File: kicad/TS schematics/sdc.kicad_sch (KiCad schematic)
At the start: 23 parts, among them J22 Activation Logic, K2 EV200-HAANA, K3 EV200-HAANA, K4 EV200-HAANA, K5 PNC113BDA, SW1 LVMS, SW10 TSMP Interlock, SW11 Motor Controller HVP800 Inter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, SW12 PL00X-301-50 Interlock, SW13 PL00Y-301-50 Interlock, SW14 PL00X-301-50 Interlock, SW15 PL00Y-301-50 Interlock, SW16 MINIMSDF000F HVD Interlock, SW2 IMD, SW3 AMS, SW5 Cockpit Shutdown Button, SW6 Left Shutdown Button, SW7 Right Shutdown Button, SW8 Inertia Switch, SW9 BOTS

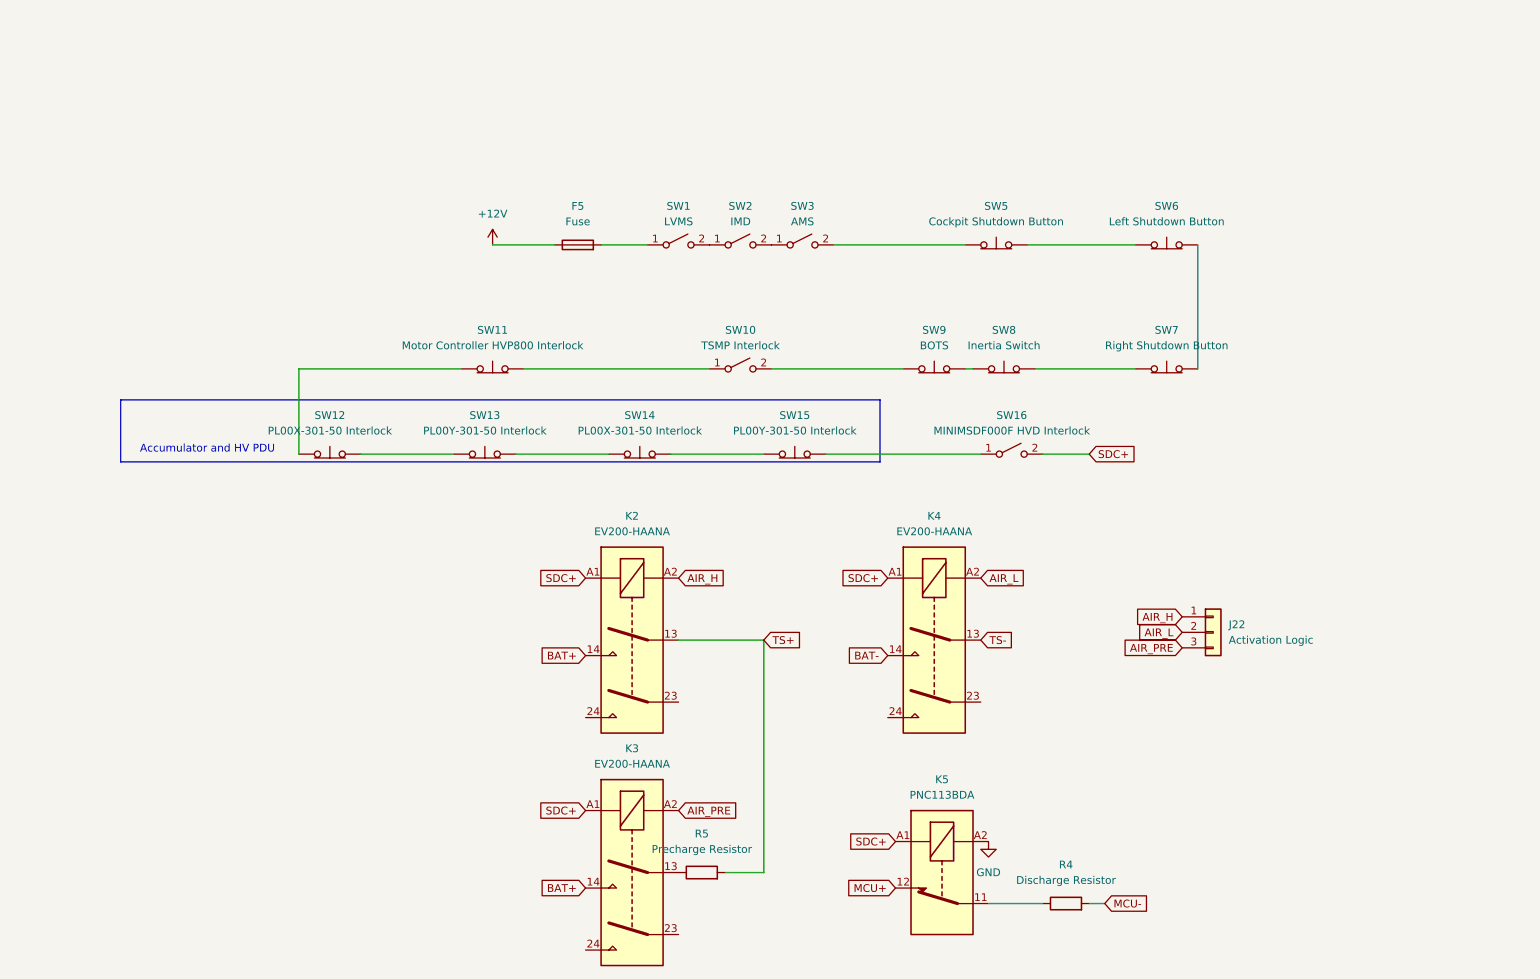
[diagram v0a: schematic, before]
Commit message: shutdown circuit
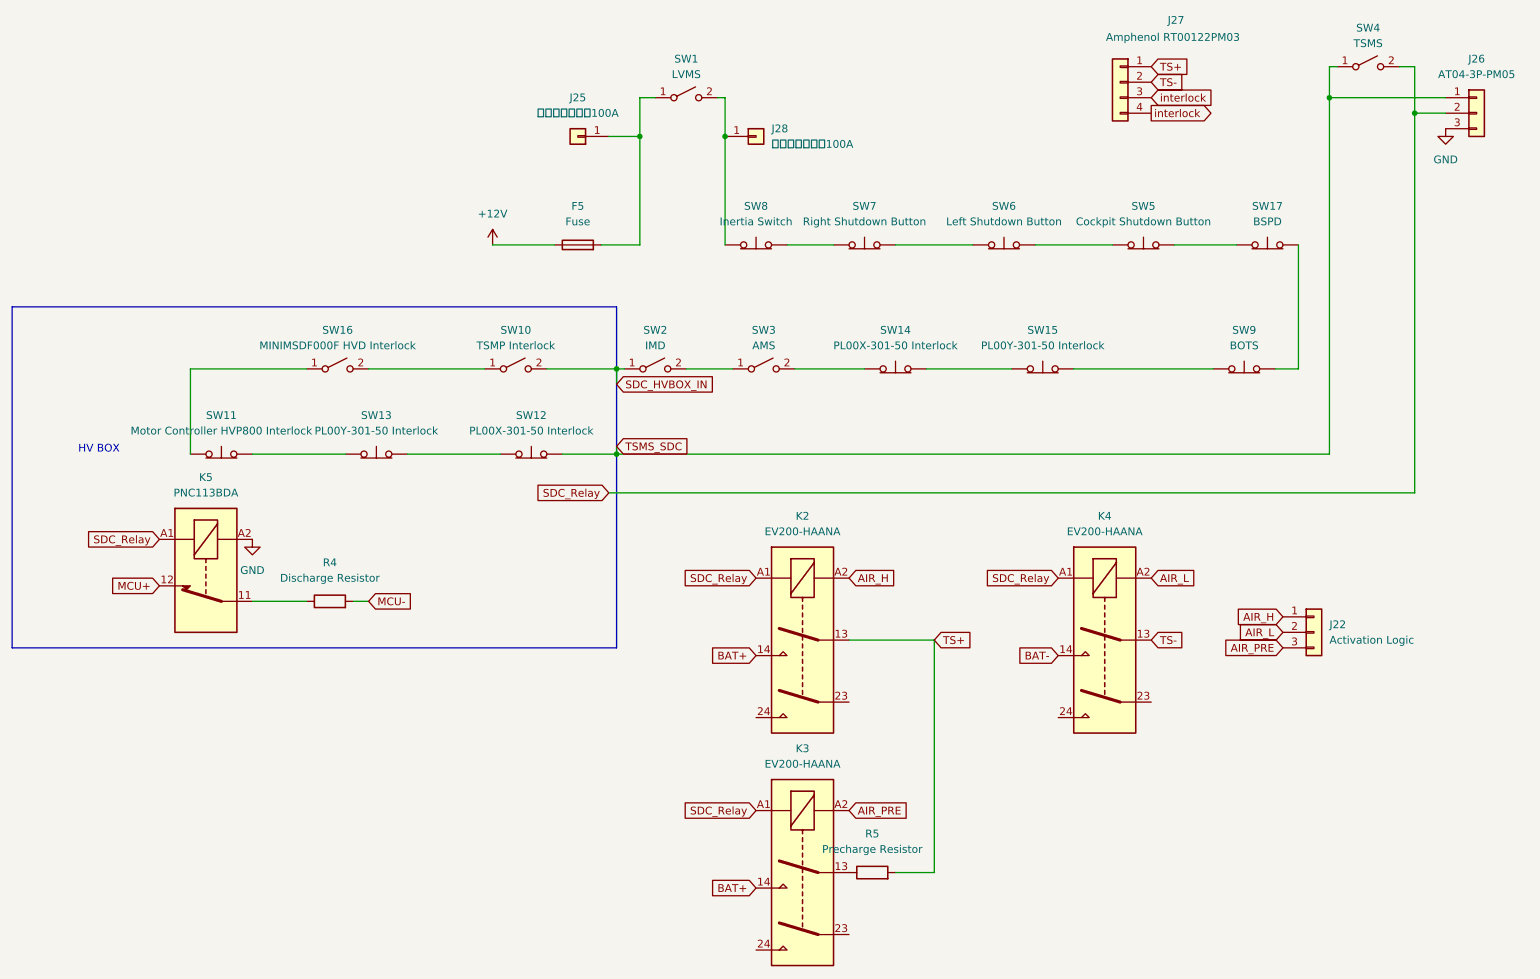
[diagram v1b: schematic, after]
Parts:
- added J25, J28: 紅色儲能接綫柱100A, symbol Connector_Generic:Conn_01x01
- added J26: AT04-3P-PM05, symbol Connector_Generic:Conn_01x03
- added J27: Amphenol RT00122PM03, symbol Connector_Generic:Conn_01x04
- added SW17: BSPD, symbol Switch:SW_Push_Open
- added SW4: TSMS, symbol Switch:SW_SPST
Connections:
- net GND: now also J26.3 (Pin_3)
- net TS+: now also J27.1 (Pin_1)
- net TS-: now also J27.2 (Pin_2)
- net at F5.2, SW1.1 (A): now also J25.1 (Pin_1)
- net at SW1.2 (B): now also SW8.1 (A), J28.1 (Pin_1); no longer SW2.1 (A)
- net at SW9.2 (B): now also SW17.2 (B); no longer SW8.1 (A)
- net at SW16.1 (A): now also SW11.1 (A); no longer SW15.2 (B)
- net at SW13.1 (A): now also SW11.2 (B); no longer SW12.2 (B)
- net at SW13.2 (B): now also SW12.1 (A); no longer SW14.1 (A)
- net at SW10.1 (A): now also SW16.2 (B); no longer SW11.2 (B)
- net at SW6.1 (A): now also SW7.2 (B); no longer SW5.2 (B)
- net at SW6.2 (B): now also SW5.1 (A); no longer SW7.2 (B)
- net at SW3.2 (B): now also SW14.1 (A); no longer SW5.1 (A)
- net at SW9.1 (A): now also SW15.2 (B); no longer SW10.2 (B)
- net SDC+ renamed SDC_Relay
- net SDC_Relay: now also J26.2 (Pin_2), SW4.2 (B); no longer SW16.2 (B)
- new net: SW17.1 (A), SW5.2 (B)
- new net SDC_HVBOX_IN: SW10.2 (B), SW2.1 (A)
- new net TSMS_SDC: J26.1 (Pin_1), SW12.2 (B), SW4.1 (A)
- new net interlock: J27.3 (Pin_3), J27.4 (Pin_4)
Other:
- note added: "HV BOX"
- note removed: "Accumulator and HV PDU"
- moved on the sheet: J22, K2, K3, K4, K5, R4, R5, SW1, SW10, SW11, SW12, SW13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

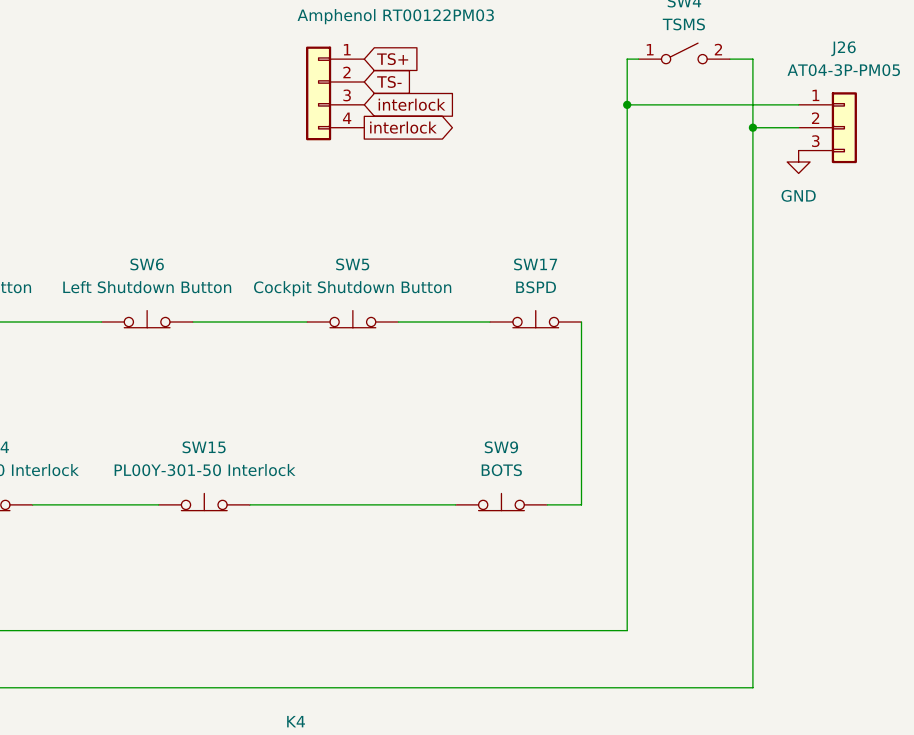
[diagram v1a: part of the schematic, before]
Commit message: haha VCU V3.2 AND NEW SCHEMATICS HAHAHA
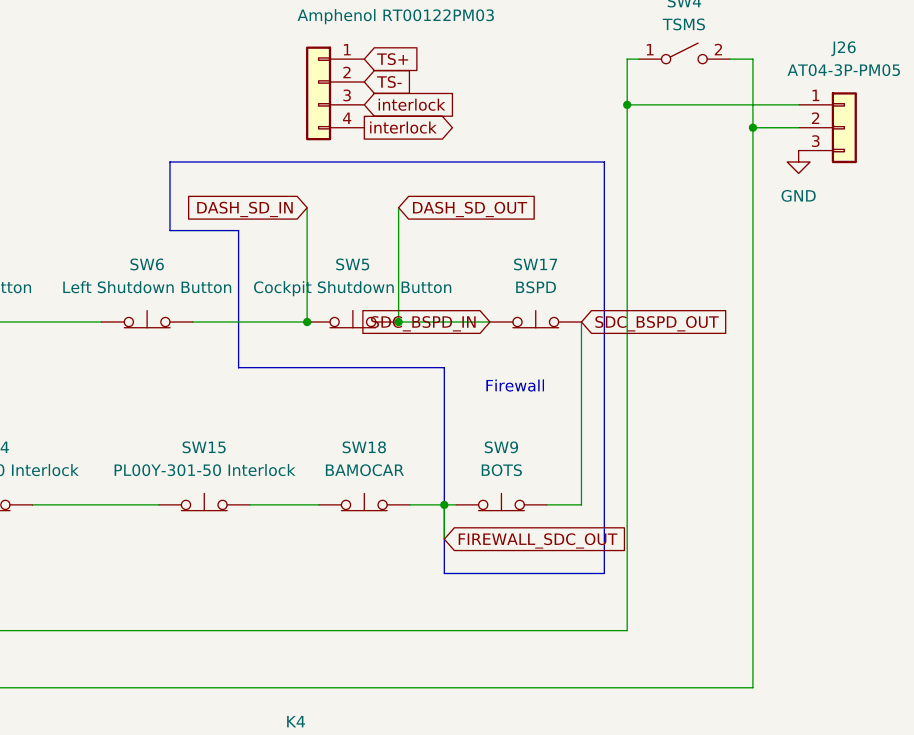
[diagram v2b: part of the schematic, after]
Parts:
- added SW18: BAMOCAR, symbol Switch:SW_Push_Open
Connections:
- net DASH_SD_IN: now reaches SW5.1 (A), SW6.2 (B)
- net DASH_SD_OUT: now reaches SW17.1 (A), SW5.2 (B)
- net SDC_BSPD_OUT: now reaches SW17.2 (B), SW9.2 (B)
- net at SW15.2 (B): now also SW18.1 (A); no longer SW9.1 (A)
- new net FIREWALL_SDC_OUT: SW18.2 (B), SW9.1 (A)
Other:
- note added: "Firewall"
